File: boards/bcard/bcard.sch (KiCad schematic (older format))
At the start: 13 parts, among them IC1 ATTINY10-TS, P1 BATT, Q1 BC846A

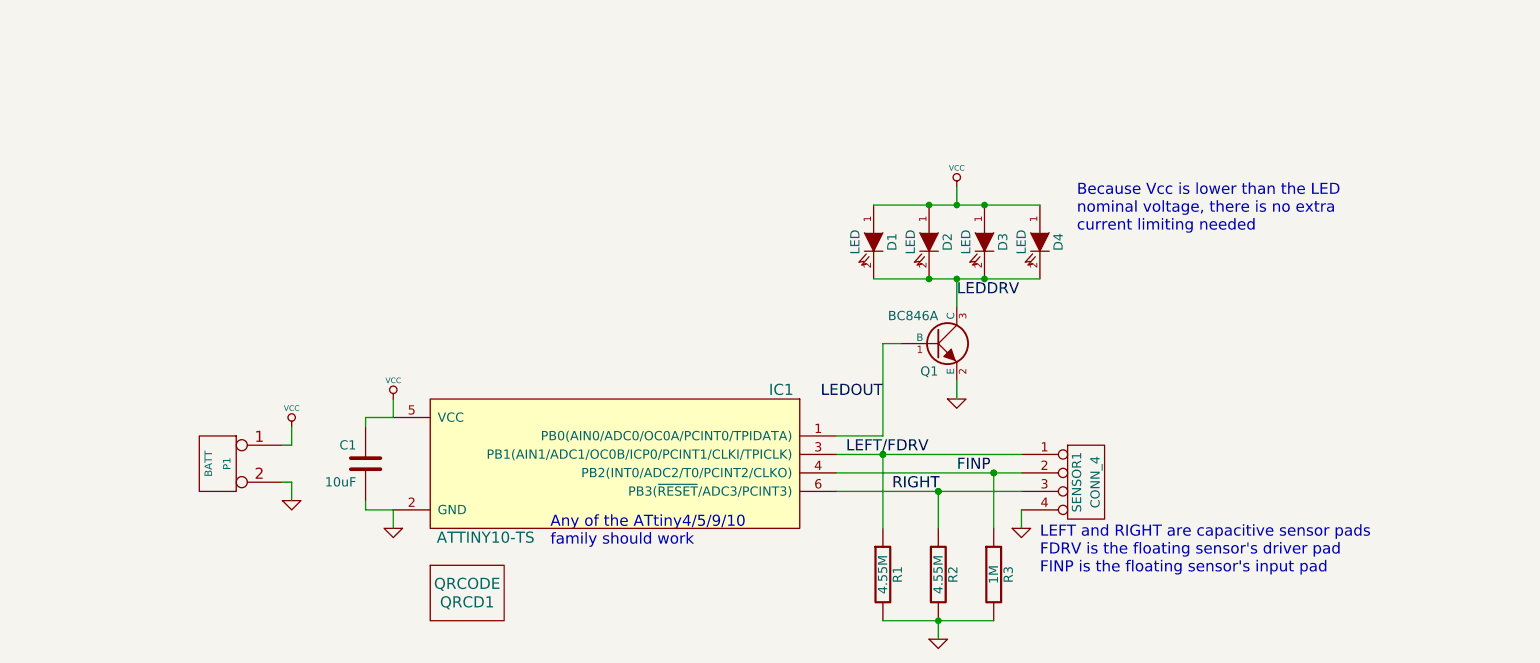
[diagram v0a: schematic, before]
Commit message: begin new phase of bcard design -- two factor auth
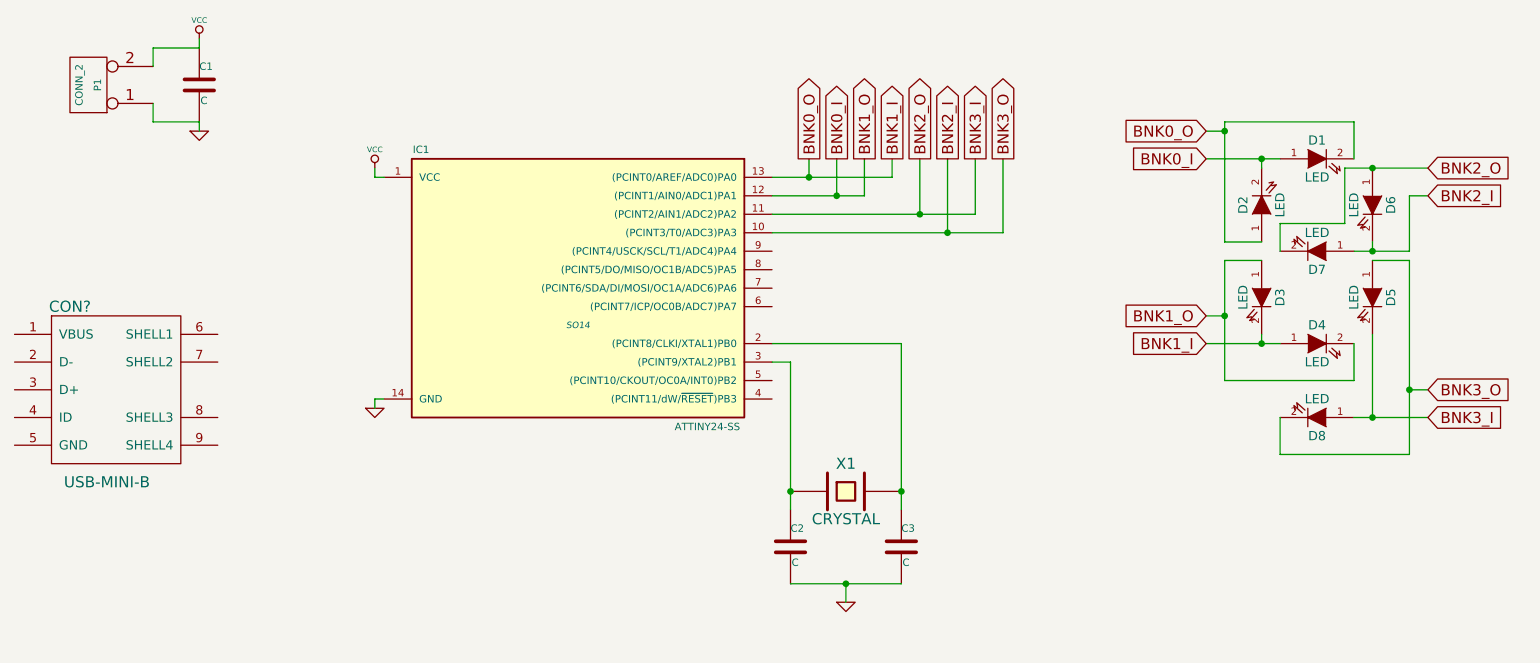
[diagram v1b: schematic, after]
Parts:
- removed IC1: ATTINY10-TS, SOT23_6, symbol ATTINY10-TS
- removed Q1: BC846A, SOT23, symbol BC846A
- removed QRCD1: QRCODE, JWCXZ, symbol LOGO
- removed R1, R2: 4.55M, SM0603, symbol R
- removed R3: 1M, SM0603, symbol R
- removed SENSOR1: CONN_4, SENSOR2, symbol CONN_4
- added C2, C3: C, symbol C
- added CON?: USB-MINI-B, symbol USB-MINI-B
- added D5, D6, D7, D8: LED, symbol LED
- added IC1: ATTINY24-SS, SO14, symbol ATTINY24-SS
- added X1: CRYSTAL, symbol CRYSTAL
- C1: value 10uF -> C; footprint SM0805 -> (none); Part GRM21BR60J106KE19L -> (none); URL http://search.digikey.com/us/en/products/GRM21BR60J106KE19L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 -> (none)
- D1, D2, D3, D4: footprint 1208vert -> (none); Part APT3216QBC/D -> (none); URL http://www.digikey.com/product-detail/en/APA3010QBC%2FD-GX/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 -> (none)
- P1: value BATT -> CONN_2; footprint 2032BATTHOLDER -> (none); Part BK-912 -> (none); URL http://www.digikey.com/product-detail/en/BK-912/BK-912-ND/2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 -> (none)
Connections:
- net GND: now also P1.1 (P1), C2.2, C3.2, IC1.14 (GND); no longer P1.2 (PM)
- net VCC: now also P1.2 (PM), IC1.1 (VCC); no longer D1.1 (A), D2.1 (A), D3.1 (A), D4.1 (A), P1.1 (P1)
- net LEDDRV renamed BNK0_I
- net BNK0_I: now also D1.1 (A), D3.1 (A), IC1.12 ((PCINT1/AIN0/ADC1)PA1); no longer D1.2 (K), D3.2 (K)
- new net: C2.1, IC1.3 ((PCINT9/XTAL2)PB1), X1.1
- new net: C3.1, IC1.2 ((PCINT8/CLKI/XTAL1)PB0), X1.2
- new net BNK0_O: D1.2 (K), D2.1 (A), D3.2 (K), D4.1 (A), IC1.13 ((PCINT0/AREF/ADC0)PA0)
- new net BNK2_I: D5.1 (A), D6.2 (K), D7.1 (A), D8.2 (K), IC1.10 ((PCINT3/T0/ADC3)PA3)
- new net BNK2_O: D5.2 (K), D6.1 (A), D7.2 (K), D8.1 (A), IC1.11 ((PCINT2/AIN1/ADC2)PA2)
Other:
- note removed: "Any of the ATtiny4/5/9/10\nfamily should work"
- note removed: "Because Vcc is lower than the LED\nnominal voltage, there is no extra\ncurrent limiting needed"
- note removed: "LEFT and RIGHT are capacitive sensor pads\nFDRV is the floating sensor's driver pad\nFINP is the floating sensor's input pad"
